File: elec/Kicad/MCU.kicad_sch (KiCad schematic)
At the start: 25 parts, among them J6 SWD, SW5 SW_Push_BOOT, SW6 SW_Push_RESET, U1 STM32L053C8T6, Y1 32MHz, Y2 32.768KHz

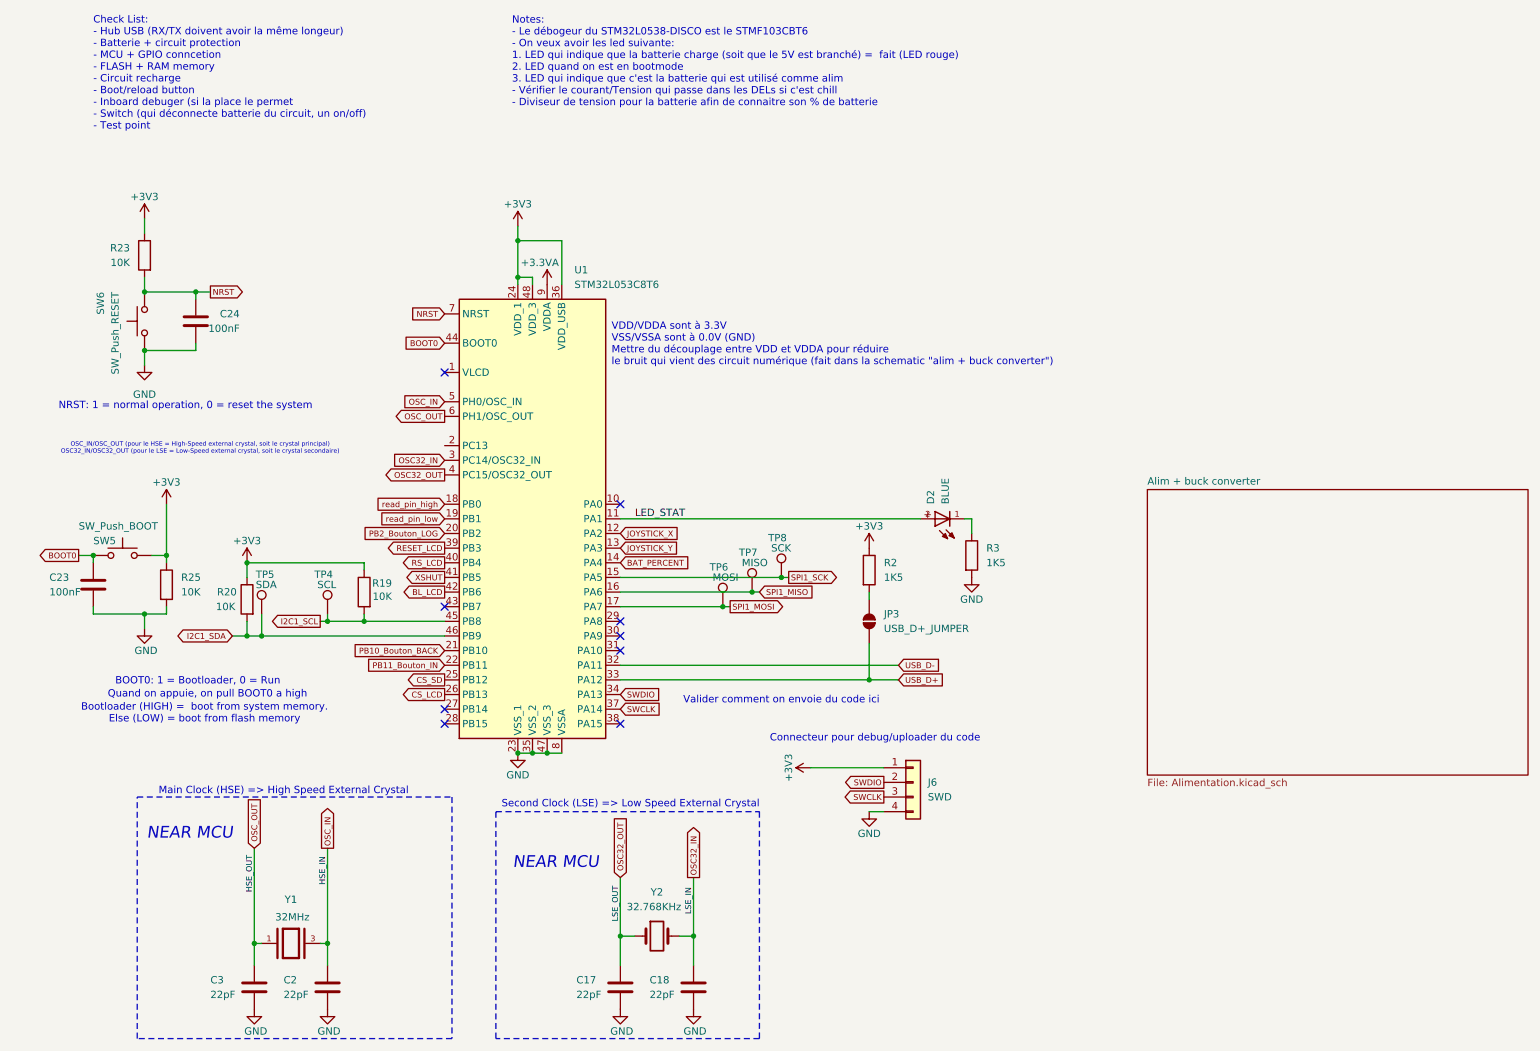
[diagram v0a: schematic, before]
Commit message: formation torture
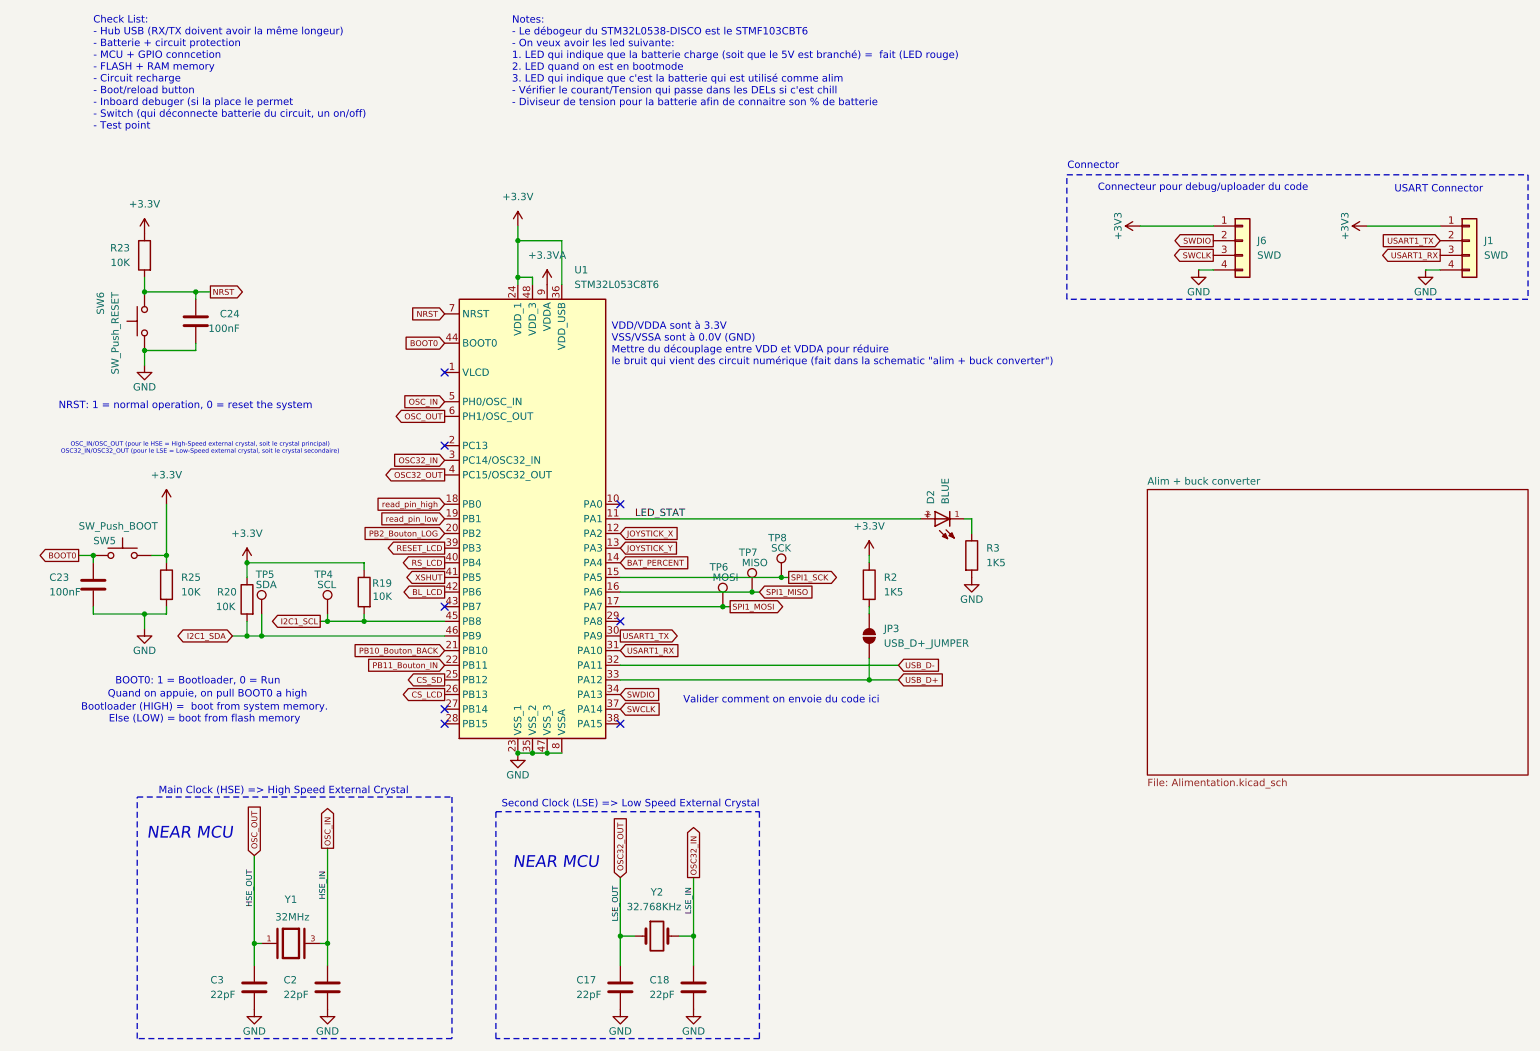
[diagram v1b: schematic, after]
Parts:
- added J1: SWD, Connector_PinHeader_2.54mm:PinHeader_1x04_P2.54mm_Vertical, symbol Connector_Generic:Conn_01x04
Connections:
- net +3V3: now also J1.1 (Pin_1); no longer R19.1, R2.1, R20.1, R23.1, R25.1, SW5.1, U1.24 (VDD_1), U1.36 (VDD_USB), U1.48 (VDD_3)
- net GND: now also J1.4 (Pin_4)
- net USART1_TX: now reaches U1.30 (PA9)
- net USART1_TX: now also J1.2 (Pin_2)
- net USART1_RX: now reaches U1.31 (PA10)
- net USART1_RX: now also J1.3 (Pin_3)
- new net +3.3V: R19.1, R2.1, R20.1, R23.1, R25.1, SW5.1, U1.24 (VDD_1), U1.36 (VDD_USB), U1.48 (VDD_3)
- no-connect marks 9 -> 8
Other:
- note added: "Connector"
- note added: "USART Connector"
- moved on the sheet: J6, JP3, R2
